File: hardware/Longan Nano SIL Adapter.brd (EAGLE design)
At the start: 49.7 x 36.8 mm, 18 parts

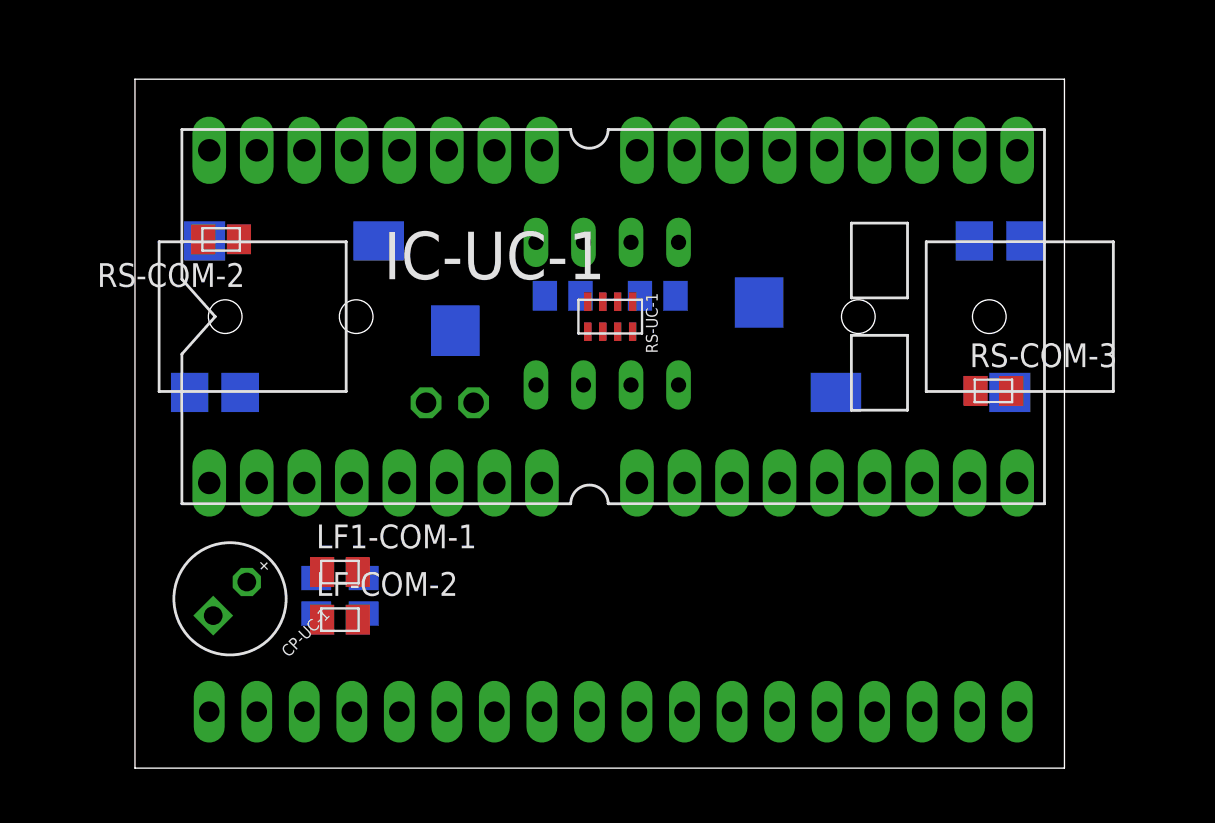
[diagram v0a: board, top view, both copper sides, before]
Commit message: final schematics and routing
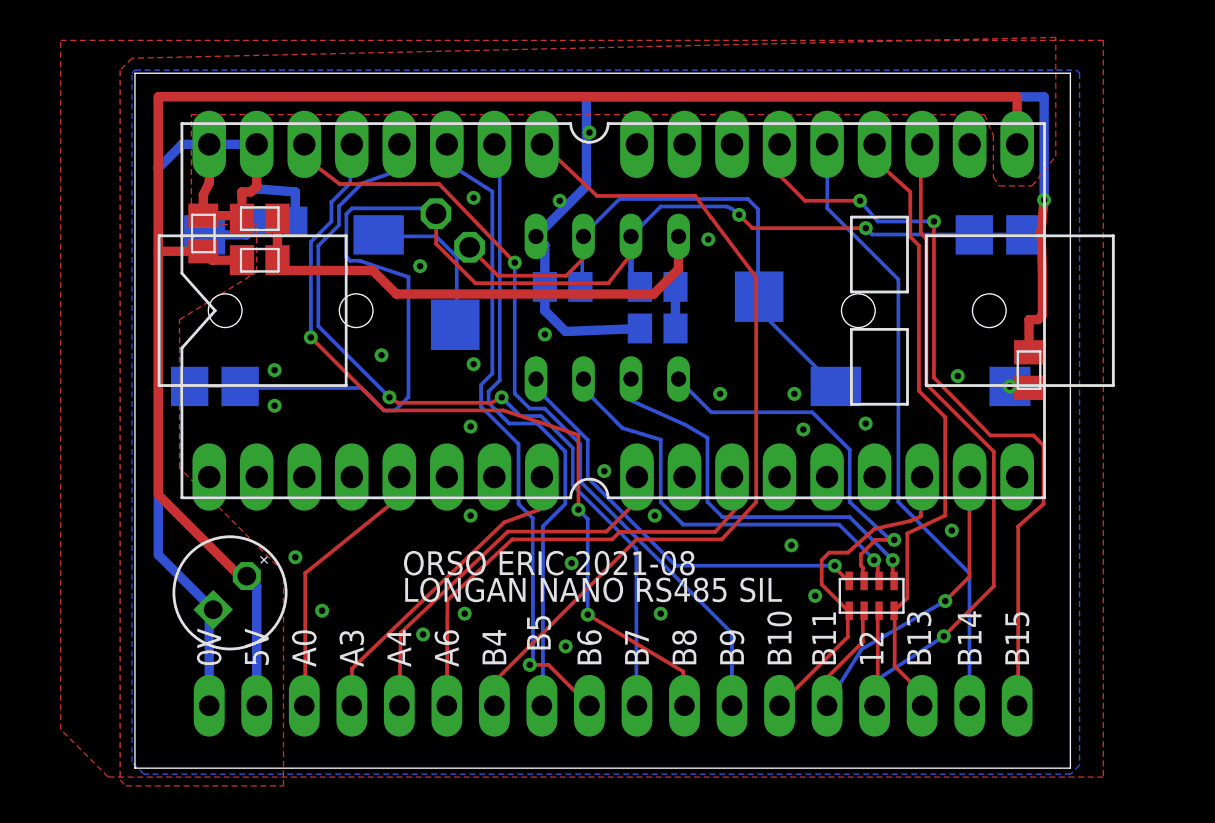
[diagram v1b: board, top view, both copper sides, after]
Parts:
- removed LF-COM-2: BEAD 500mA, 2021-07-02 OrangeHat Library:SMD-M2012
- added CB-COM-1: 1u, Passives:SMD-M2012
- added U$1: (no value), Library:SIGNATURE_ADROBOT_SMALL
- added U$2: (no value), Library:SIGNATURE_ORANGEBOT_SMALL
- CF-COM-1: value 100n 50v -> 100n; device 2021-07-02 OrangeHat Library:SMD-M2012 -> Passives:SMD-M2012
- CF-COM-2: value 100n 50V -> 100n; device 2021-07-02 OrangeHat Library:SMD-M2012 -> Passives:SMD-M2012
- CON-COM-1, CON-COM-2: device 2021-07-02 OrangeHat Library:JACK_SMD_3MM5 -> Library:JACK_SMD_3MM5
- LF1-COM-1, RS-COM-2, RS-COM-3: device 2021-07-02 OrangeHat Library:SMD-M2012 -> Passives:SMD-M2012
- RS-UC-1: value RX4-M2012-X4 -> 4X1K
- moved CF-COM-2 20.9 mm to (6.67, 29.4), flipped to the top, turned to 0 degrees
- moved RS-UC-1 20.4 mm to (39.4, 9.21), turned to 0 degrees
- moved CF-COM-1 20.3 mm to (3.65, 28.6), flipped to the top, turned to 270 degrees
- moved LF1-COM-1 17.2 mm to (6.67, 27.1)
- moved RT-COM-1 9.21 mm to (17.0, 28.7), turned to 45 degrees
- moved RS-COM-2 3.16 mm to (7.62, 29.2), flipped to the bottom, turned to 0 degrees
- moved RS-COM-3 2.21 mm to (47.8, 21.3), turned to 270 degrees
- moved RD-COM-1 0.48 mm to (22.9, 25.7)
- moved RU-COM-1 0.48 mm to (27.9, 25.7)
- moved CON-COM-1 0.32 mm to (8.57, 24.4)
- moved CON-COM-2 0.32 mm to (41.9, 24.4)
- moved IC-UC-1 0.32 mm to (24.3, 24.4)
- moved CP-UC-1 0.32 mm to (5.08, 9.37)
- moved CON-UC-1 0.32 mm to (2.70, 3.33)
- moved CON-UC-2 0.32 mm to (7.78, 3.33)
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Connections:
- removed net V-485: CF-COM-2.1, IC-COM-1.5, LF-COM-2.2, RD-COM-1.1, RS-COM-2.1, RS-COM-3.1
- net V+485: now also CB-COM-1.2
- net V-: now also CB-COM-1.1, CF-COM-2.1, IC-COM-1.5, RD-COM-1.1, RS-COM-2.1, RS-COM-3.1; no longer LF-COM-2.1
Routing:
- net V-: track 0.00 -> 136.1 mm, vias 0 -> 30
- net V+: track 0.00 -> 88.1 mm
- net CHB485: track 0.00 -> 69.7 mm, vias 0 -> 2
- net UC-PB4: track 0.00 -> 46.1 mm
- net UC-PB8: track 0.00 -> 44.9 mm, vias 0 -> 3
- net UC-PB7: track 0.00 -> 43.7 mm, vias 0 -> 2
- net UC-PB9: track 0.00 -> 43.0 mm, vias 0 -> 1
- net CHA485: track 0.00 -> 42.0 mm
- net UC-PB15: track 0.00 -> 41.3 mm, vias 0 -> 2
- net UC-PB12: track 0.00 -> 39.9 mm, vias 0 -> 1
- net UC-PB6: track 0.00 -> 34.6 mm, vias 0 -> 1
- net UC-PB13: track 0.00 -> 33.8 mm
- net UC-PB5: track 0.00 -> 33.5 mm
- net UC-PB14: track 0.00 -> 33.2 mm
- net V+485: track 0.00 -> 31.8 mm
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- added copper zone on layer 1, net V+
- added copper zone on layer 1, net V-
- added copper zone on layer 16, net V-
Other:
- board size 49.7 x 36.8 mm -> 50 x 37.1 mm
- board text added: "0V"
- board text added: "12"
- board text added: "120"
- board text added: "5V"
- board text added: "A0"
- board text added: "A3"
- board text added: "A4"
- board text added: "A6"
- board text added: "B10"
- board text added: "B11"
- board text added: "B12"
- board text added: "B13"
- board text added: "B14"
- board text added: "B15"
- board text added: "B4"
- board text added: "B5"
- board text added: "B6"
- board text added: "B7"
- board text added: "B8"
- board text added: "B9"
- board text added: "LONGAN NANO RS485 SIL"
- board text added: "ORSO ERIC 2021-08"
